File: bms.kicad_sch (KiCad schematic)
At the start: 19 parts, among them Q1 SSM6K513NU-LF, Q2 SSM6K513NU-LF, Q3 2N7002W, U1 BQ28Z620DRZR

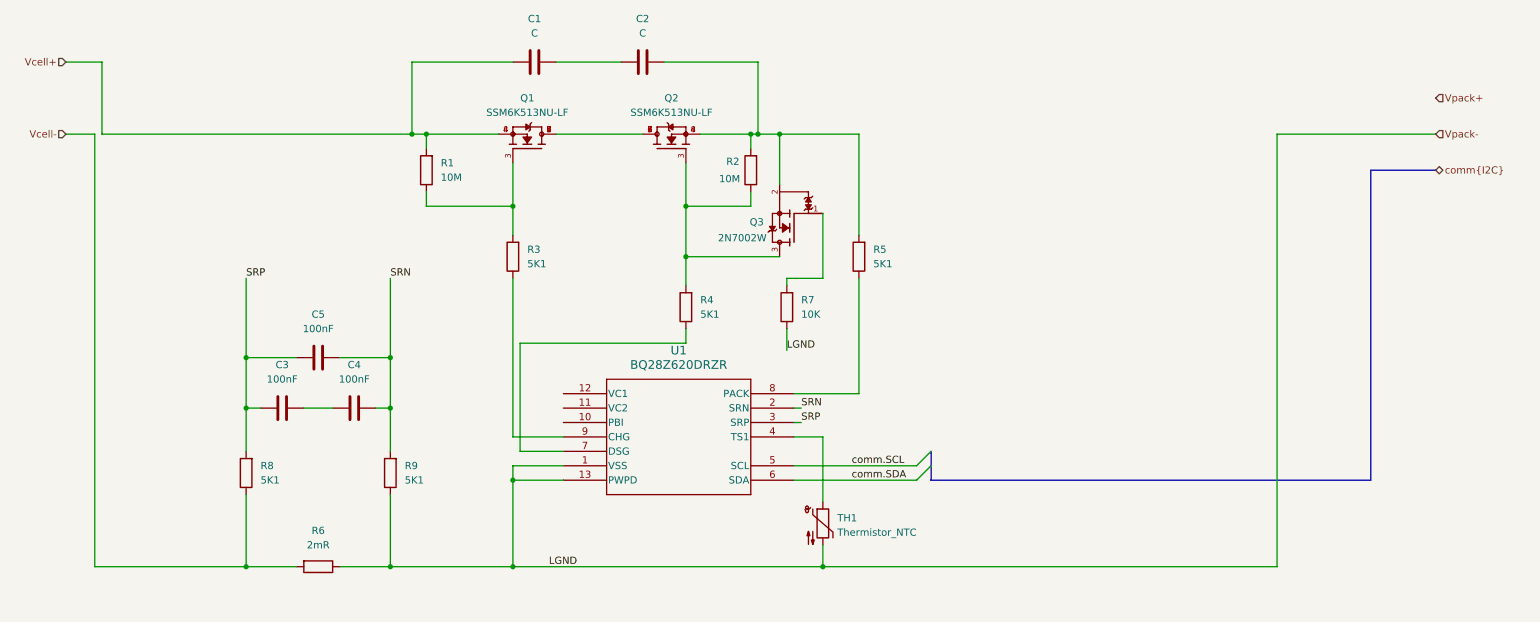
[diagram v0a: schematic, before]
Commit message: Batter scematic done.
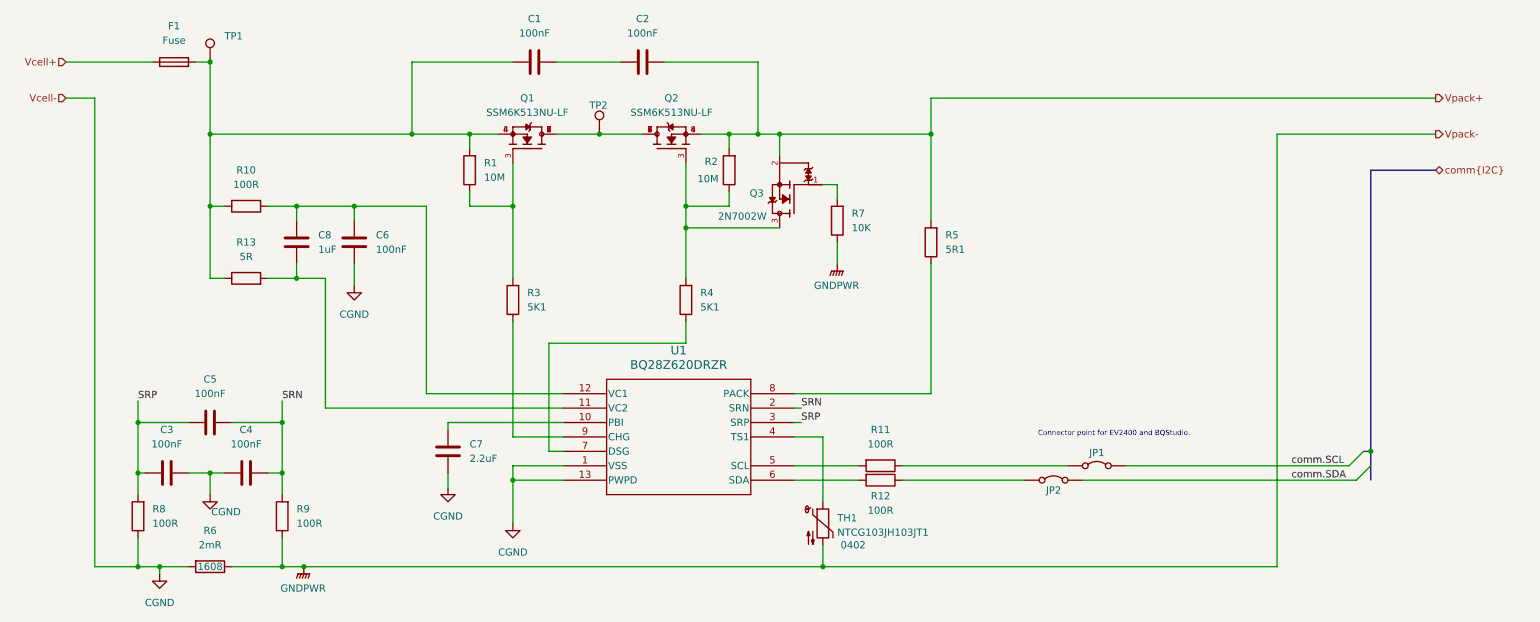
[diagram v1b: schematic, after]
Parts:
- added C6: 100nF, Capacitor_SMD:C_0603_1608Metric_Pad1.08x0.95mm_HandSolder, symbol Device:C
- added C7: 2.2uF, Capacitor_SMD:C_0603_1608Metric_Pad1.08x0.95mm_HandSolder, symbol Device:C
- added C8: 1uF, Capacitor_SMD:C_0603_1608Metric_Pad1.08x0.95mm_HandSolder, symbol Device:C
- added F1: Fuse, Resistor_SMD:R_0603_1608Metric_Pad0.98x0.95mm_HandSolder, symbol Device:Fuse
- added JP1, JP2: Jumper_2_Bridged, Connector_PinHeader_2.54mm:PinHeader_1x02_P2.54mm_Horizontal, symbol Jumper:Jumper_2_Bridged
- added R10, R11, R12: 100R, Resistor_SMD:R_0603_1608Metric_Pad0.98x0.95mm_HandSolder, symbol Device:R
- added R13: 5R, Resistor_SMD:R_0603_1608Metric_Pad0.98x0.95mm_HandSolder, symbol Device:R
- added TP1, TP2: TestPoint, TestPoint:TestPoint_Pad_D1.5mm, symbol Connector:TestPoint
- C1, C2: value C -> 100nF
- R5: value 5K1 -> 5R1
- R6: Size (none) -> 1608; Tolerance (none) -> 1%
- R8, R9: value 5K1 -> 100R
- TH1: value Thermistor_NTC -> NTCG103JH103JT1; Size (none) -> 0402
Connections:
- net Vcell- is gone; now on net CGND: R6.2, R8.1
- net Vcell+: now also F1.1; no longer C1.1, Q1.4, Q1.8, R1.2
- net Vpack+: now also C2.2, Q2.4, Q2.8, Q3.2, R2.2, R5.2
- net comm.SCL: now also JP1.2 (B); no longer U1.5 (SCL)
- net comm.SDA: now also JP2.2 (B); no longer U1.6 (SDA)
- net at Q1.1, Q1.2, Q1.5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: now also TP2.1
- net CGND: now reaches C3.2, C4.1
- net CGND: now also U1.1 (VSS), U1.13 (PWPD), C6.1, C7.1
- net at U1.10 (PBI): now also C7.2
- net at U1.11 (VC2): now also C8.1, R13.2
- net at U1.12 (VC1): now also C6.2, C8.2, R10.1
- net Vpack- renamed GNDPWR
- net GNDPWR: no longer U1.1 (VSS), U1.13 (PWPD)
- new net: C1.1, F1.2, Q1.4, Q1.8, R1.2, R10.2, R13.1, TP1.1
- new net: JP1.1 (A), R11.1
- new net: R11.2, U1.5 (SCL)
- new net: JP2.1 (A), R12.1
- new net: R12.2, U1.6 (SDA)
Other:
- note added: "Connector point for EV2400 and BQStudio."
- moved on the sheet: C3, C4, C5, Q3, R1, R2, R3, R4, R5, R6, R7, R8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

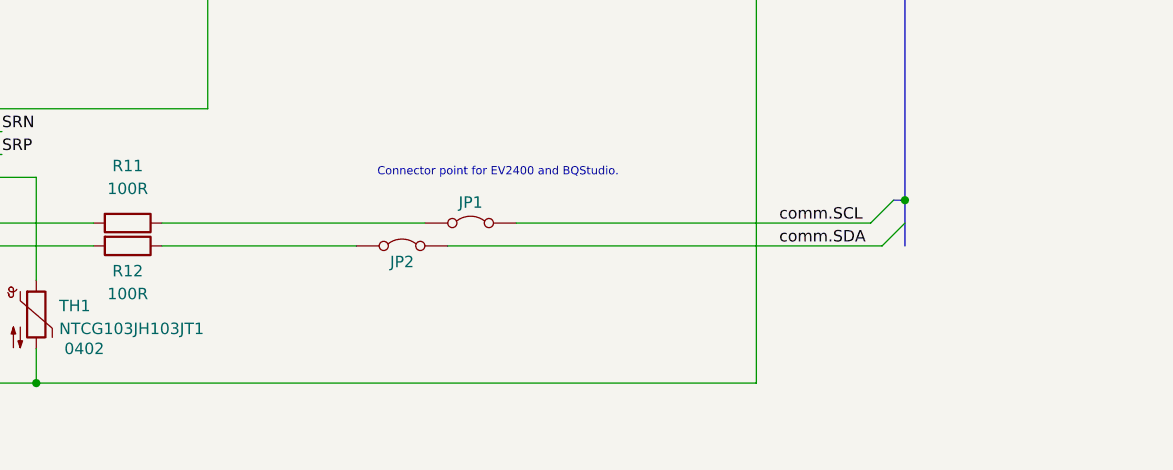
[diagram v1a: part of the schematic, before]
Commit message: Draw power schematic.
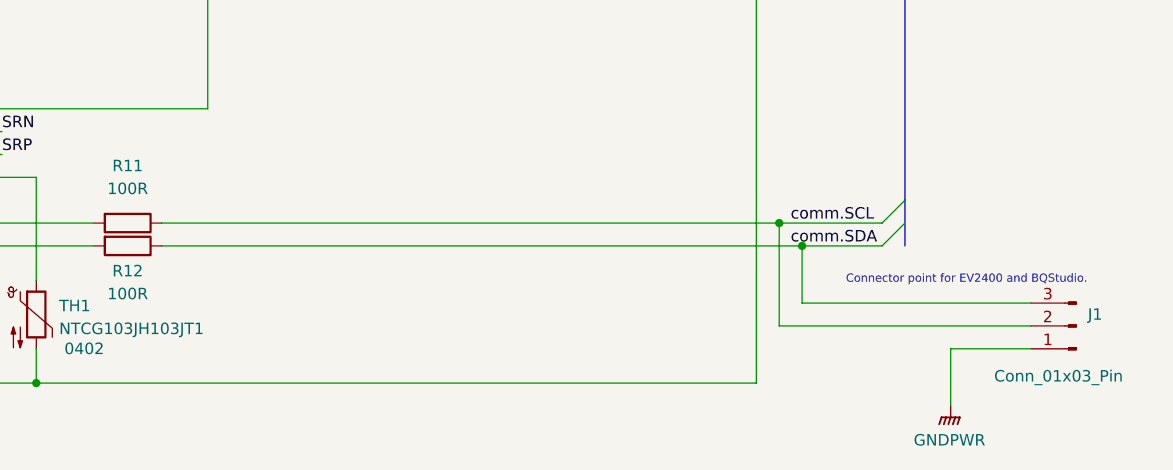
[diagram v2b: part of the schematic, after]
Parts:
- removed JP1, JP2: Jumper_2_Bridged, Connector_PinHeader_2.54mm:PinHeader_1x02_P2.54mm_Horizontal, symbol Jumper:Jumper_2_Bridged
- added J1: Conn_01x03_Pin, Connector_PinHeader_2.54mm:PinHeader_1x03_P2.54mm_Horizontal, symbol Connector:Conn_01x03_Pin
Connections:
- net GNDPWR: now also J1.1 (Pin_1)
- net comm.SCL: now also R11.1, J1.2 (Pin_2)
- net comm.SDA: now also R12.1, J1.3 (Pin_3)
